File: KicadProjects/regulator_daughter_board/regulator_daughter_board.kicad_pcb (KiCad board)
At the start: 2 copper layers, 7 parts, among them J1 Conn_01x04, U1 TPS613222ADBVR

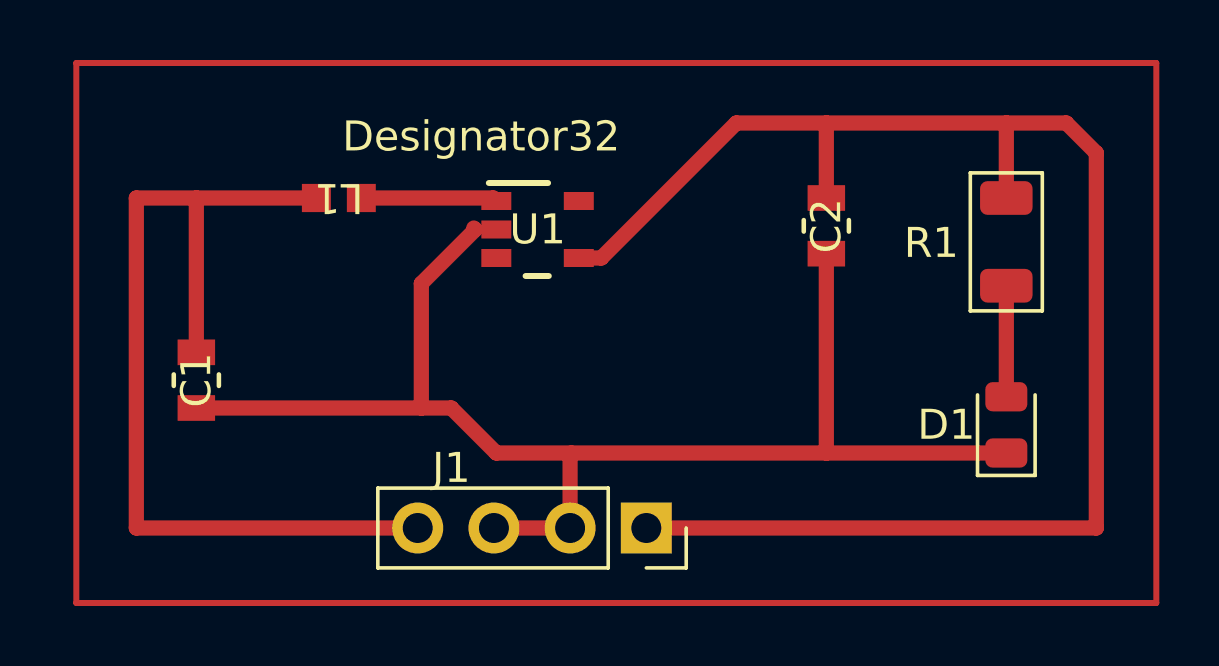
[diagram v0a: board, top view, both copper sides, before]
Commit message: yup
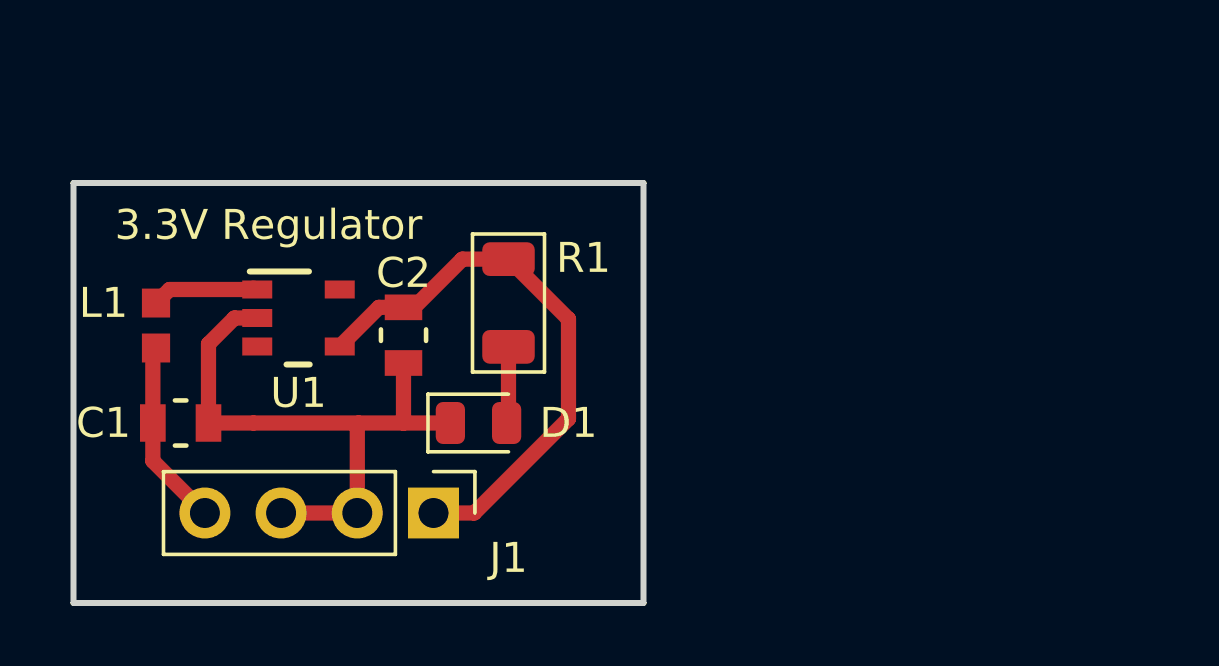
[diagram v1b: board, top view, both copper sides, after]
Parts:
- J1: footprint Connector_PinSocket_2.54mm:PinSocket_1x04_P2.54mm_Vertical -> Connector_PinHeader_2.54mm:PinHeader_1x04_P2.54mm_Vertical
- moved D1 17.6 mm to (13.4, -6.00), turned to 0 degrees
- moved R1 16.7 mm to (14.4, -10.0)
- moved C2 14.6 mm to (10.9, -8.93)
- moved U1 8.50 mm to (7.41, -9.50)
- moved L1 7.43 mm to (2.66, -9.25), turned to -90 degrees
- moved J1 7.11 mm to (11.9, -3.00)
- moved C1 1.52 mm to (3.48, -6.00), turned to 180 degrees
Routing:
- net /Vout: track 52.0 -> 18.8 mm
- net GNDPWR: track 46.8 -> 20.2 mm
- net /Vin: track 31.6 -> 6.47 mm
- net Net-(D1-A): track 3.70 -> 2.06 mm
- net Net-(U1-SW): track 4.54 -> 3.56 mm
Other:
- board outline added: 19 x 14 mm
